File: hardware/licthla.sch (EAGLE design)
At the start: 8 parts, among them U1 NCP1117LPST50T3G

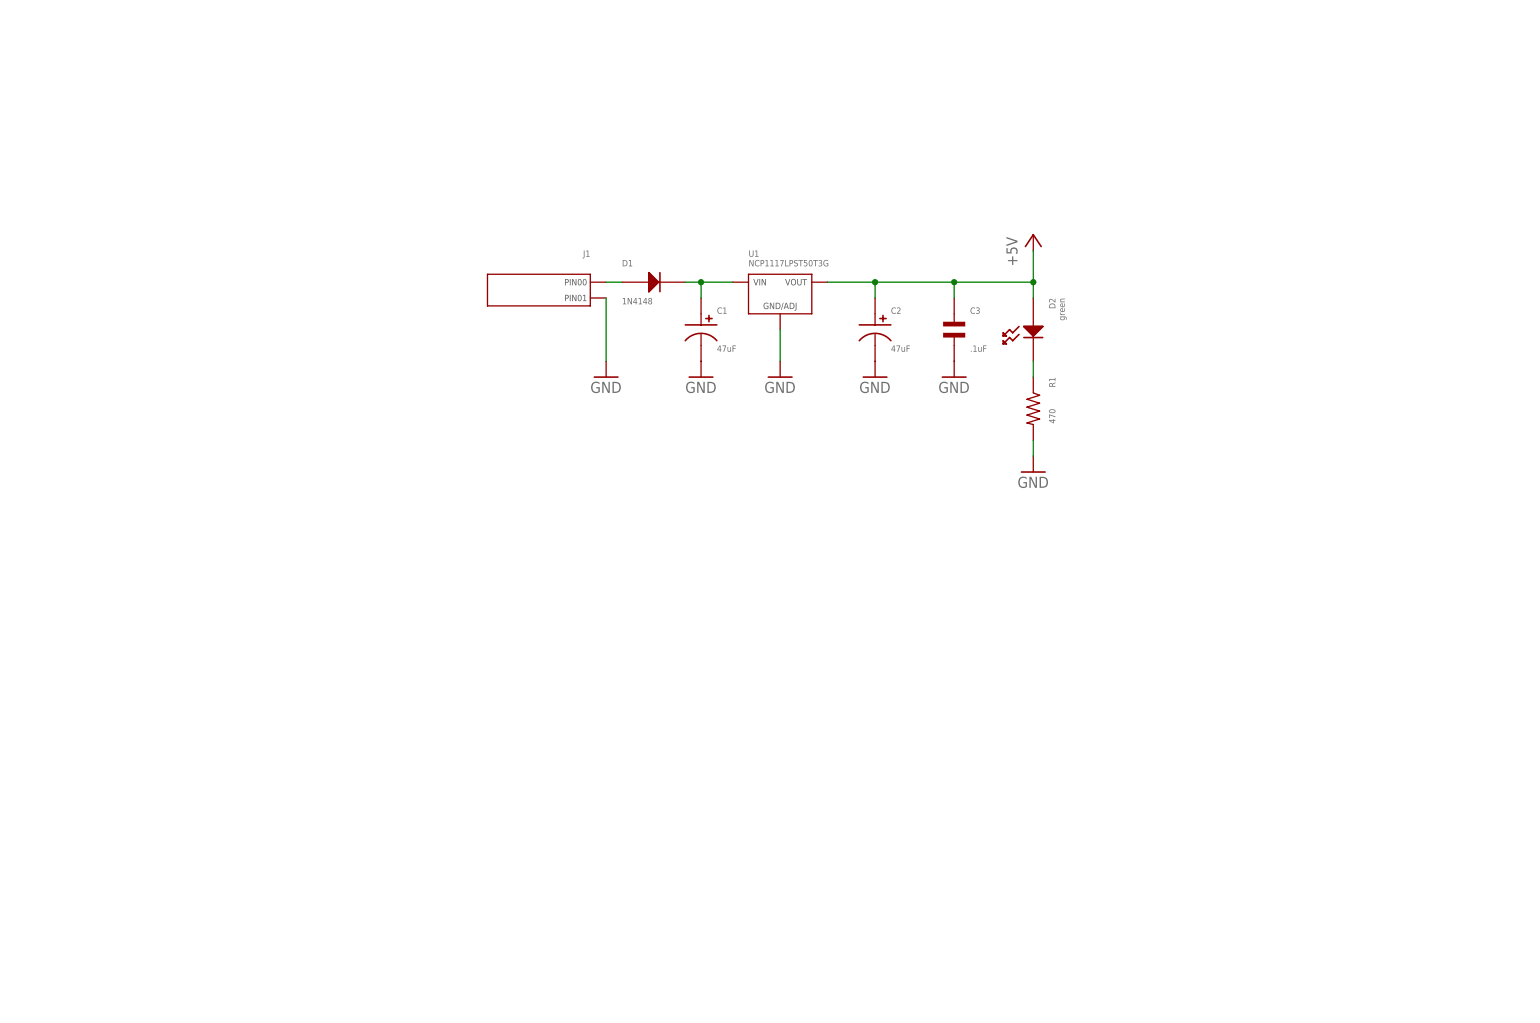
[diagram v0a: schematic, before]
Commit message: Some more work on the AVR part of the schematic
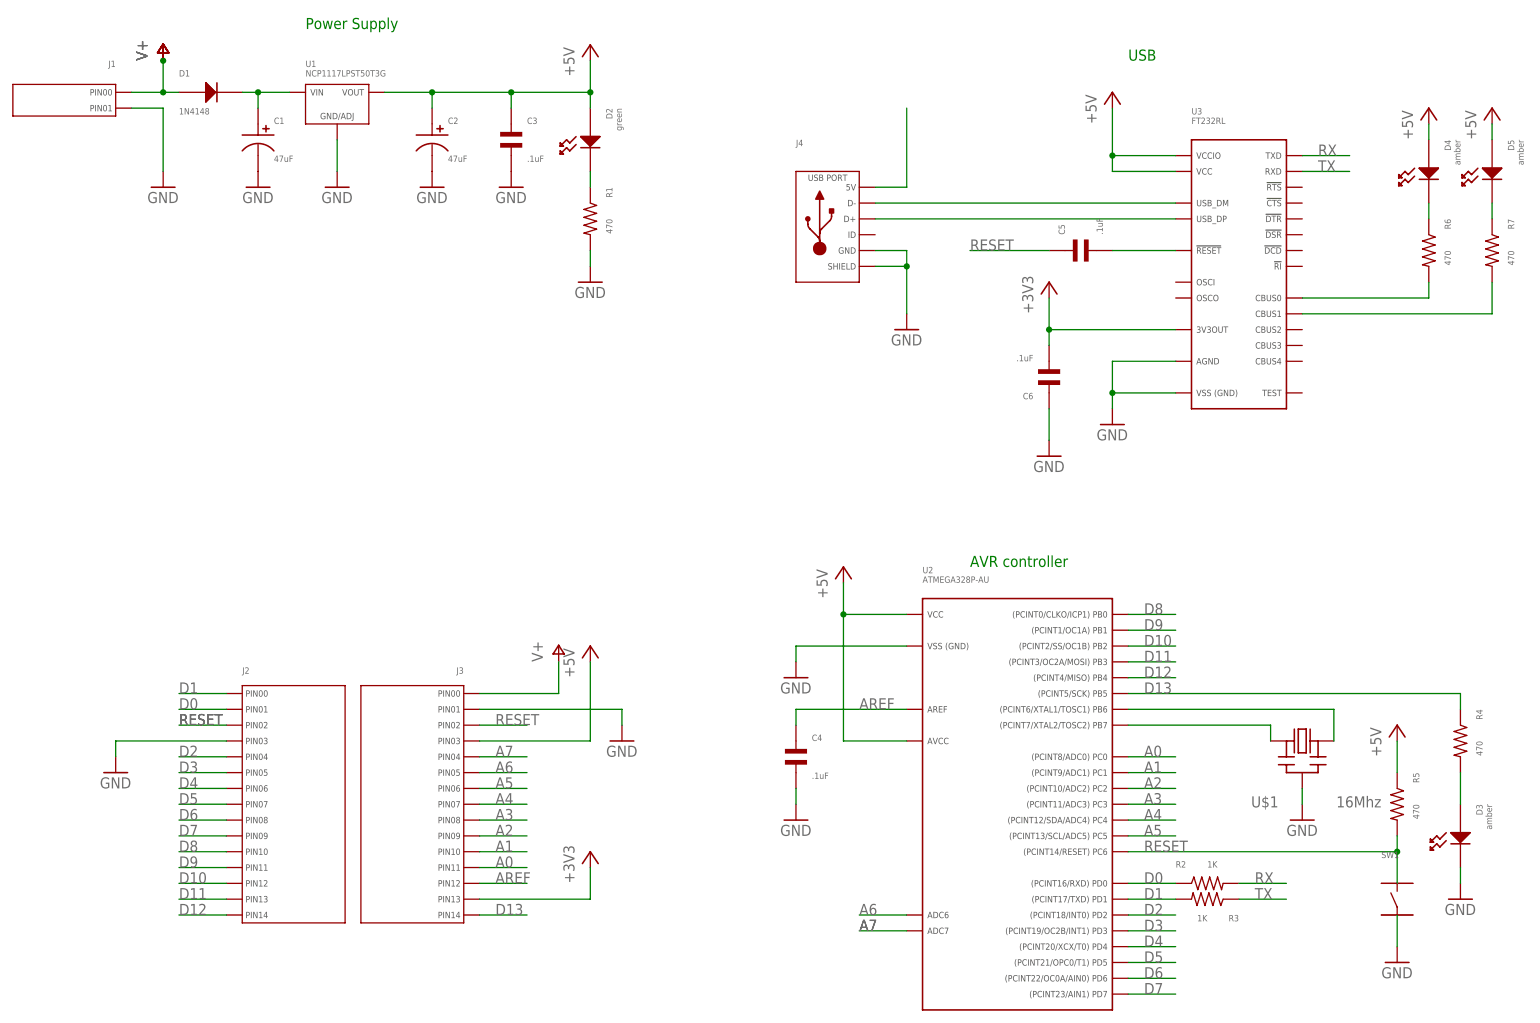
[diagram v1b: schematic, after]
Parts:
- added C4, C5, C6: .1uF, MF_Passives:CAPACITOR_NP_0402
- added D3, D4, D5: amber, MF_LEDs:LED_SINGLE_0805
- added J2, J3: (no value), MF_Connectors:HEADER_01X15_PTH_2.54MM
- added J4: (no value), MF_Connectors:USB_MICRO_RIGHT
- added R2, R3: 1K, MF_Passives:RESISTOR_0805
- added R4, R5, R6, R7: 470, MF_Passives:RESISTOR_0805
- added SW1: (no value), MF_Switches:TACT_6MM
- added U$1: 16Mhz, adafruit:CERMOSCILL-AWCSR
- added U2: ATMEGA328P-AU, MF_IC_Digital:ATMEGA328P-AU
- added U3: FT232RL, MF_IC_Digital:FT232RL
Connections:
- new net +3V3: C6.P$2, J3.PIN13, U3.3V3OUT
- new net A0: J3.PIN11, U2.PC0
- new net A1: J3.PIN10, U2.PC1
- new net A2: J3.PIN9, U2.PC2
- new net A3: J3.PIN8, U2.PC3
- new net A4: J3.PIN7, U2.PC4
- new net A5: J3.PIN6, U2.PC5
- new net A6: J3.PIN5, U2.ADC6
- new net A7: J3.PIN4, U2.ADC7
- new net AREF: C4.P$1, J3.PIN12, U2.AREF
- new net D0: J2.PIN1, R2.P$1, U2.PD0
- new net D1: J2.PIN0, R3.P$2, U2.PD1
- new net D10: J2.PIN12, U2.PB2
- new net D11: J2.PIN13, U2.PB3
- new net D12: J2.PIN14, U2.PB4
- new net D13: J3.PIN14, R4.P$1, U2.PB5
- new net D2: J2.PIN4, U2.PD2
- new net D3: J2.PIN5, U2.PD3
- new net D4: J2.PIN6, U2.PD4
- new net D5: J2.PIN7, U2.PD5
- new net D6: J2.PIN8, U2.PD6
- new net D7: J2.PIN9, U2.PD7
- new net D8: J2.PIN10, U2.PB0
- new net D9: J2.PIN11, U2.PB1
- new net N$11: D4.CATHODE, R6.P$1
- new net N$12: D5.CATHODE, R7.P$1
- new net N$13: R6.P$2, U3.CBUS0
- new net N$14: R7.P$2, U3.CBUS1
- new net N$2: J4.D-, U3.USBDM
- new net N$5: U$1.IN, U2.PB7
- new net N$6: U$1.OUT, U2.PB6
- new net N$7: D3.ANODE, R4.P$2
- new net N$8: C5.P$2, U3.!RESET
- new net RESET: C5.P$1, J2.PIN2, J3.PIN2, R5.P$2, U2.PC6
- new net RX: R2.P$2, U3.TXD
- new net TX: R3.P$1, U3.RXD
- new net V+: D1.ANODE, J1.PIN0, J3.PIN0
- new net VUSB: J4.5V
- net +5V: now also D4.ANODE, D5.ANODE, J3.PIN3, R5.P$1, U2.AVCC, U2.VCC, U3.VCC, U3.VCCIO
- net GND: now also C4.P$2, C6.P$1, D3.CATHODE, J2.PIN3, J3.PIN1, J4.GND, J4.SLD, U$1.GND, U2.GND, U3.AGND, U3.GND
- net N$3: now also J4.D+, U3.USBDP; no longer D1.ANODE, J1.PIN0
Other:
- note added: "AVR controller"
- note added: "Power Supply"
- note added: "USB"
- moved on the sheet: C1, C2, C3, D1, D2, J1, R1, U1
